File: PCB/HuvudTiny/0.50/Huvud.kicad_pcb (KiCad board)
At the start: 4 copper layers, 42 x 42 mm, 113 parts, among them J1 Conn_02x02_Odd_Even, J12 USB_Micro-B_Molex-105017-0001, J2 DBG, J3 THERM, J4 FAN0, J5 FAN1, J6 Heater, J7 Endstop, J9 STEPPER, Q1 AO3400A, Q2 AO3400A, Q3 AON7524, U2 TMC2209-LA, U3 TPS54308, U5 STM32F103C8T6, U6 SN65HVD230, Y1 8Mhz

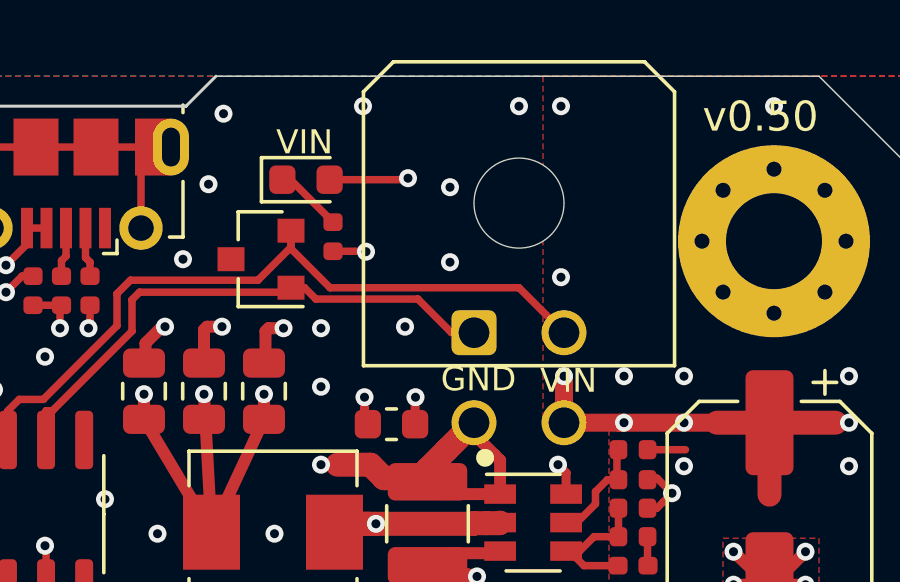
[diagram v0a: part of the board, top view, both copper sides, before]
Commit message: 0.50 huvud
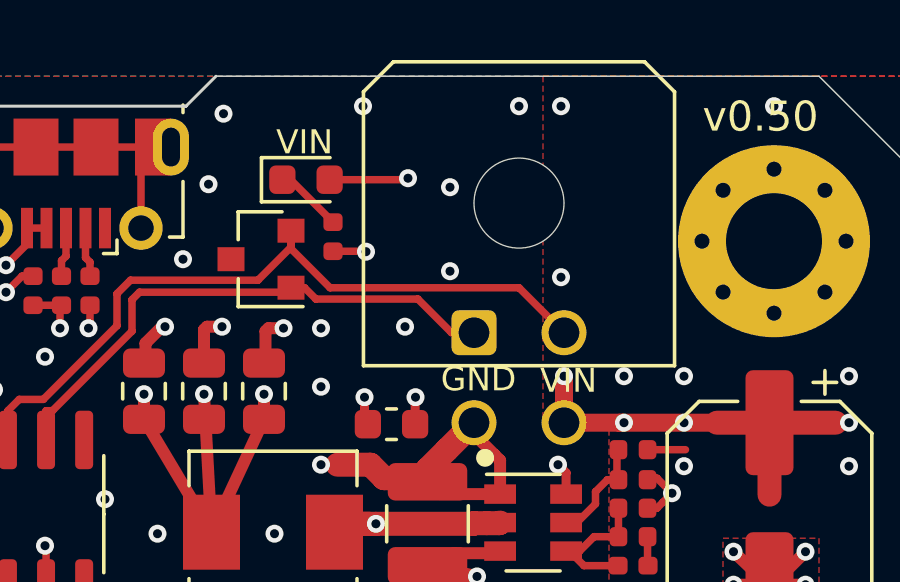
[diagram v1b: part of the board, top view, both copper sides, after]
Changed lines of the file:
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@@
   (segment (start 193.6 105.0625) (end 193.6 105.6) (width 0.25) (layer F.Cu) (net 2))
   (segment (start 193.6 105.6) (end 192.9 106.3) (width 0.25) (layer F.Cu) (net 2))
-  (via (at 207.7 106.2) (size 0.6) (drill 0.3) (layers F.Cu B.Cu) (net 2))
+  (via (at 207.7 106.5) (size 0.6) (drill 0.3) (layers F.Cu B.Cu) (net 2))
   (via (at 215.1 113.9) (size 0.6) (drill 0.3) (layers F.Cu B.Cu) (net 2))
   (segment (start 214.800001 114.199999) (end 215.1 113.9) (width 0.25) (layer F.Cu) (net 2))
